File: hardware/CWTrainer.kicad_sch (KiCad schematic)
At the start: 22 parts, among them J1 Analog, J2 Digital, J3 CW Out, J4 CW paddle in, J5 Headphones, J6 CW Paddle out, Q1 BC547, SW5 CW Paddle, U1 LCD1602-I2C, U2 pam8403

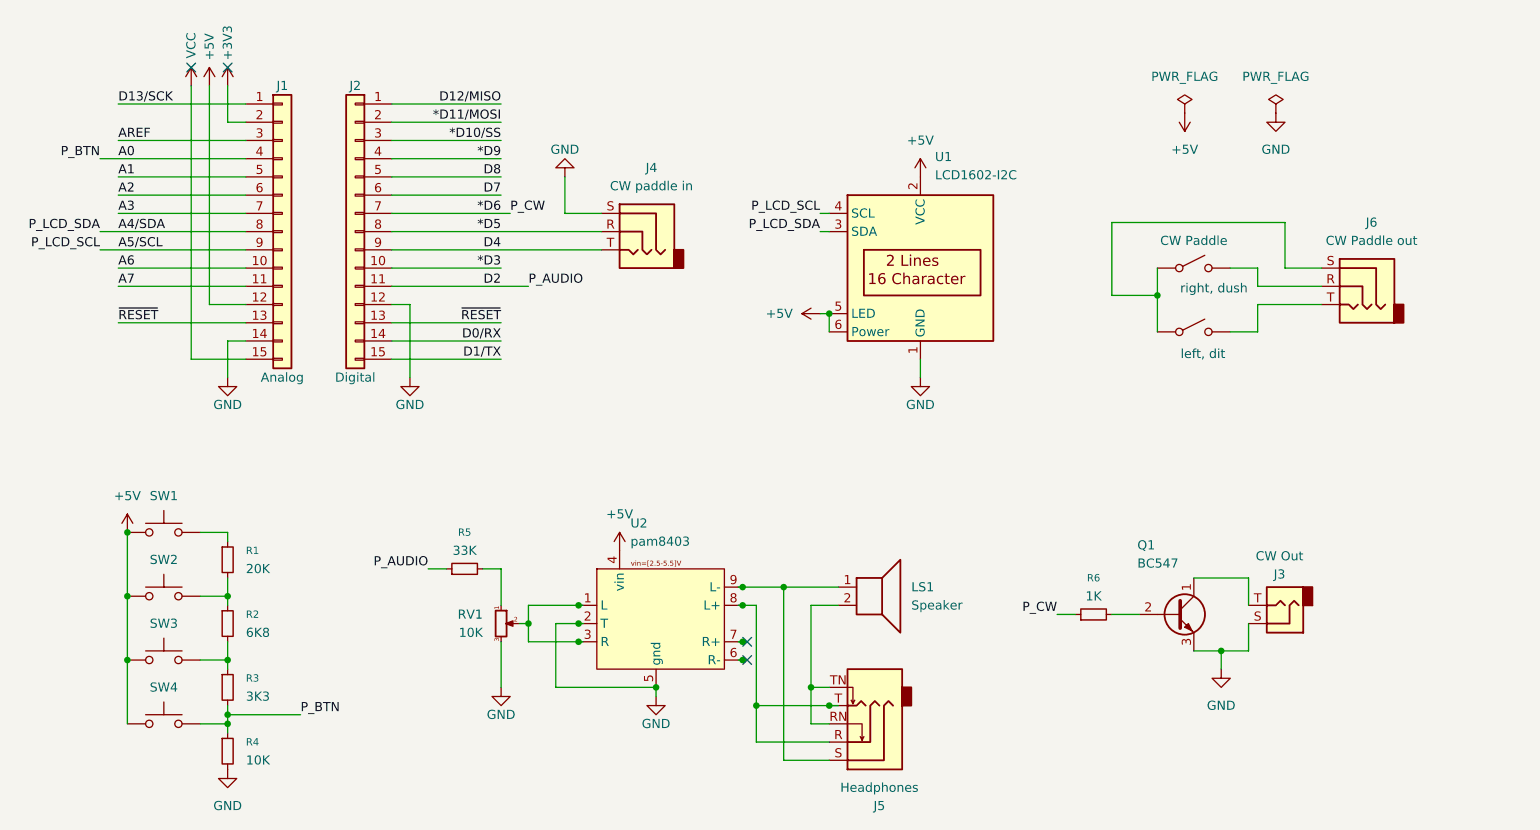
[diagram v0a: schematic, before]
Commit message: 0.95 RC2
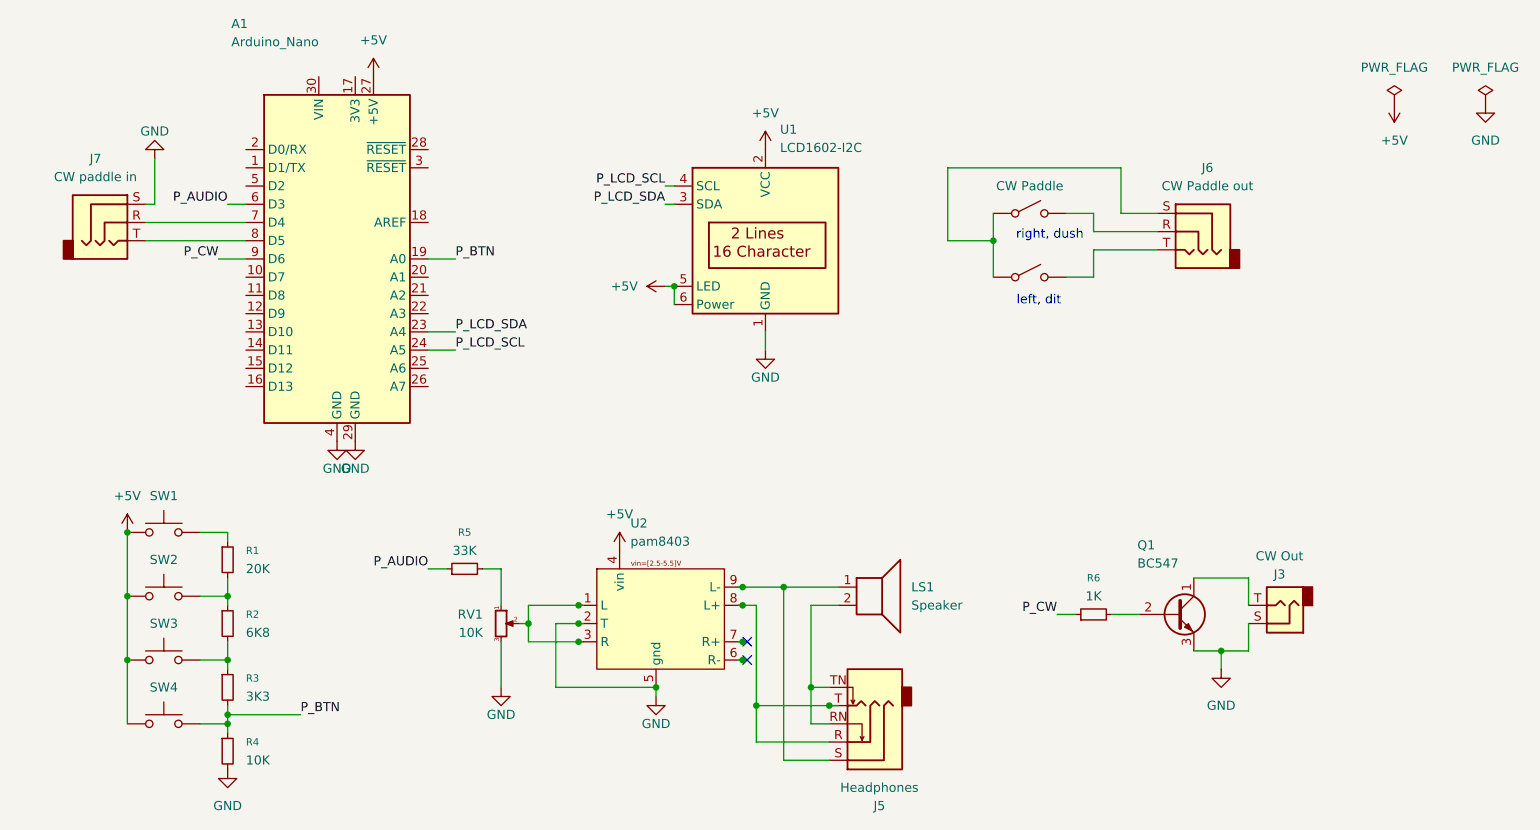
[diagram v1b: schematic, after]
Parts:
- removed J1: Analog, Connector_PinHeader_2.54mm:PinHeader_1x15_P2.54mm_Vertical, symbol Connector_Generic:Conn_01x15
- removed J2: Digital, Connector_PinHeader_2.54mm:PinHeader_1x15_P2.54mm_Vertical, symbol Connector_Generic:Conn_01x15
- removed J4: CW paddle in, symbol Connector_Audio:AudioJack3
- added A1: Arduino_Nano, Module:Arduino_Nano, symbol MCU_Module:Arduino_Nano_v3.x
- added J7: CW paddle in, symbol Connector_Audio:AudioJack3
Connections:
- net +5V: now also A1.27 (+5V)
- net GND: now also A1.29 (GND), A1.4 (GND), J7.S
- net *D6 renamed P_CW
- net P_CW: now also A1.9 (D6)
- net A0 renamed P_BTN
- net P_BTN: now also A1.19 (A0)
- net A4/SDA renamed P_LCD_SDA
- net P_LCD_SDA: now also A1.23 (A4)
- net A5/SCL renamed P_LCD_SCL
- net P_LCD_SCL: now also A1.24 (A5)
- net D2 renamed P_AUDIO
- net P_AUDIO: now also A1.6 (D3)
- new net: A1.7 (D4), J7.R
- new net: A1.8 (D5), J7.T
- no-connect marks 4 -> 2
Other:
- moved on the sheet: J6, U1
